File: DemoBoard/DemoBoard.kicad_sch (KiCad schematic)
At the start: 58 parts, among them J1 USB4110GFA, J2 Conn_01x10_Pin, J3 Conn_01x10_Pin, J4 Conn_01x10_Pin, J5 Conn_01x10_Pin, SW1 SW_Push, SW2 SW_Push, U1 RP2040, U2 W25Q128JVSIM, U3 MCP2518FDT-E_QBB, U4 TCAN332DCNR, U5 TLV75533PDBVR, Y1 ABM8-272-T3, Y2 ABM8-20.000MHZ-10-B1U-T

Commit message: Merging v0.1 to main (#1)
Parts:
- removed J2, J3, J4, J5: Conn_01x10_Pin, Connector_PinSocket_2.54mm:PinSocket_1x10_P2.54mm_Vertical, symbol Connector:Conn_01x10_Pin
- removed JP1: 3, Jumper:SolderJumper-2_P1.3mm_Open_RoundedPad1.0x1.5mm, symbol Jumper:SolderJumper_2_Open
- removed JP2: 2, Jumper:SolderJumper-2_P1.3mm_Open_RoundedPad1.0x1.5mm, symbol Jumper:SolderJumper_2_Open
- removed JP3: 1, Jumper:SolderJumper-2_P1.3mm_Open_RoundedPad1.0x1.5mm, symbol Jumper:SolderJumper_2_Open
- removed JP4: 0, Jumper:SolderJumper-2_P1.3mm_Open_RoundedPad1.0x1.5mm, symbol Jumper:SolderJumper_2_Open
- added C24: 100nF, Capacitor_SMD:C_0402_1005Metric_Pad0.74x0.62mm_HandSolder, symbol Device:C
- added C25: 47uF, Capacitor_SMD:C_1206_3216Metric_Pad1.33x1.80mm_HandSolder, symbol Device:C
- added J6: M55-7101242R, inspireFly:HARWIN_M55-7101242R, symbol inspireFly:M55-7101242R
- added J7: MSD-1-A, inspireFly:CUI_MSD-1-A, symbol inspireFly:MSD-1-A
- added J8: Conn_01x17_Pin, Connector_PinSocket_2.54mm:PinSocket_1x17_P2.54mm_Vertical, symbol Connector:Conn_01x17_Pin
- added R11: 10k, Resistor_SMD:R_0402_1005Metric_Pad0.72x0.64mm_HandSolder, symbol Device:R_US
- C22: footprint Capacitor_SMD:C_0402_1005Metric -> Capacitor_SMD:C_0402_1005Metric_Pad0.74x0.62mm_HandSolder
- C23: value 10uF -> 47uF; footprint Capacitor_SMD:C_0402_1005Metric -> Capacitor_SMD:C_1206_3216Metric_Pad1.33x1.80mm_HandSolder
- JP5: value SolderJumper_2_Open -> 3.3V EN; footprint Jumper:SolderJumper-2_P1.3mm_Open_RoundedPad1.0x1.5mm -> inspireFly:SmallJumper
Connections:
- net +3.3V: now also C24.1, J6.B1, J6.B2, J6.B3, J7.4 (VDD), J8.3 (Pin_3), R11.1
- net ADC_0: now also J8.8 (Pin_8)
- net ADC_1: now also J8.9 (Pin_9)
- net ADC_2: now also J8.10 (Pin_10)
- net ADC_3: now also J8.11 (Pin_11)
- net CAN_HIGH: now also J6.A1, J8.2 (Pin_2)
- net CAN_LOW: now also J6.A2, J8.1 (Pin_1)
- net GPIO_14: now also J8.13 (Pin_13)
- net GPIO_15: now also J8.14 (Pin_14)
- net GPIO_16: now also J8.15 (Pin_15)
- net GPIO_17: now also J8.16 (Pin_16)
- net GPIO_6: now also R8.1
- net GPIO_9: now also J8.12 (Pin_12)
- net SPI0_CLK: now also J7.5 (CLK)
- net SPI0_MISO: now also J7.7 (DAT0)
- net SPI0_MOSI: now also J7.3 (CMD)
- net SWCLK: now also J8.4 (Pin_4)
- net SWD: now also J8.6 (Pin_6)
- net VBUS: now also J8.7 (Pin_7)
- net GND renamed COVER_GND
- net COVER_GND: now also C24.2, C25.2, J6.A3, J6.A4, J6.A5, J6.A6, J6.SH1, J6.SH2, J6.SH3, J6.SH4, J7.6 (VSS), J7.G1 (COVER_GND), J7.G2 (COVER_GND), J7.G3 (COVER_GND), J7.G4 (COVER_GND), J8.17 (Pin_17), J8.5 (Pin_5)
- net GPIO_5_DEBUGLED renamed SPI0_CS_SDCARD
- net SPI0_CS_SDCARD: now also J7.2 (CD/DAT3), R11.2; no longer R8.1
- net SPI0_CS renamed SPI0_CS_CAN
- new net BATTERY_VOLTAGE: C25.1, J6.B4, J6.B5, J6.B6
- no-connect marks 5 -> 8
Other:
- note added: "4.2V max voltage"
- note added: "Board Connector"
- note added: "Debug LEDs"
- note added: "Ground unused ADC pins"
- note added: "SD Card"
- note added: "Test Pinout"
- note removed: "Debug + Pinout"
- note removed: "Ground by soldering jumper if not using ADC pin"
- moved on the sheet: C12, C16, C23, CR1, D1, D2, J1, R1, R6, R7, R8, R9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

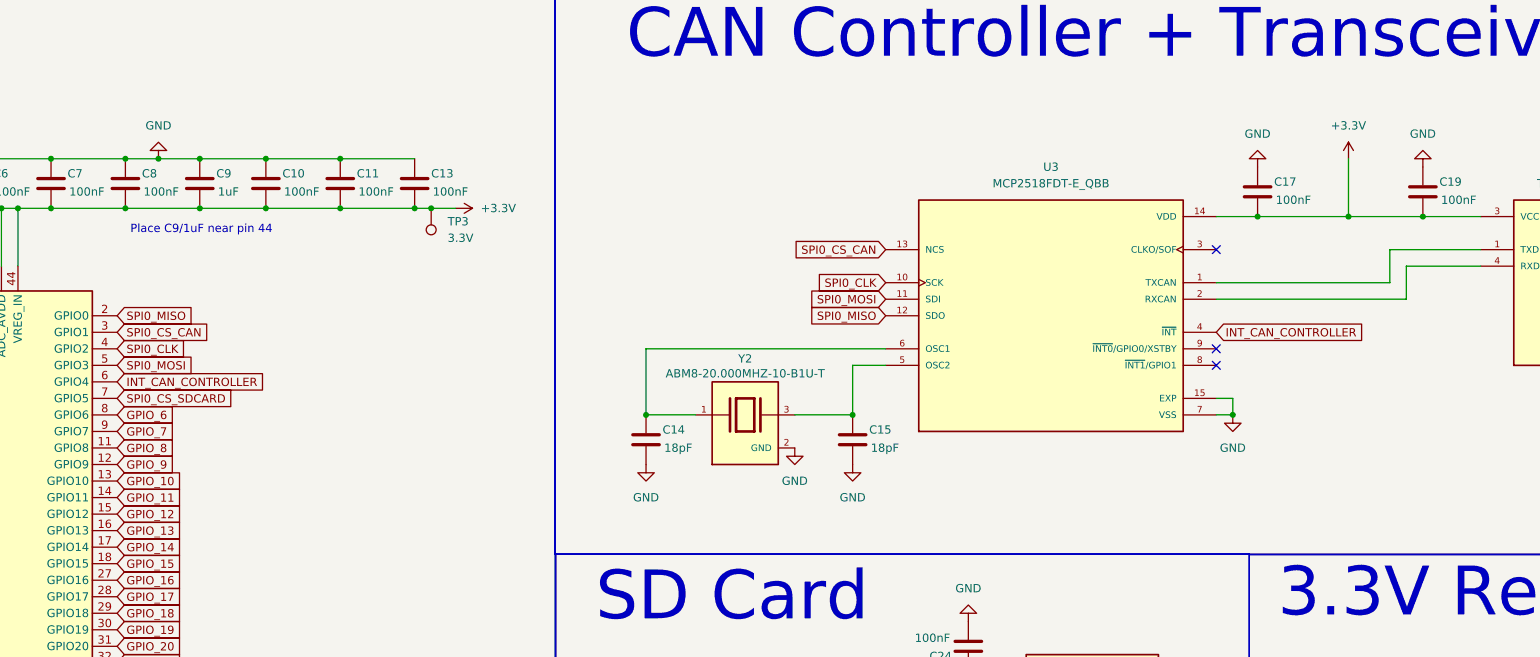
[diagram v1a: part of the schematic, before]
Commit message: Updated DemoBoard to V0.2
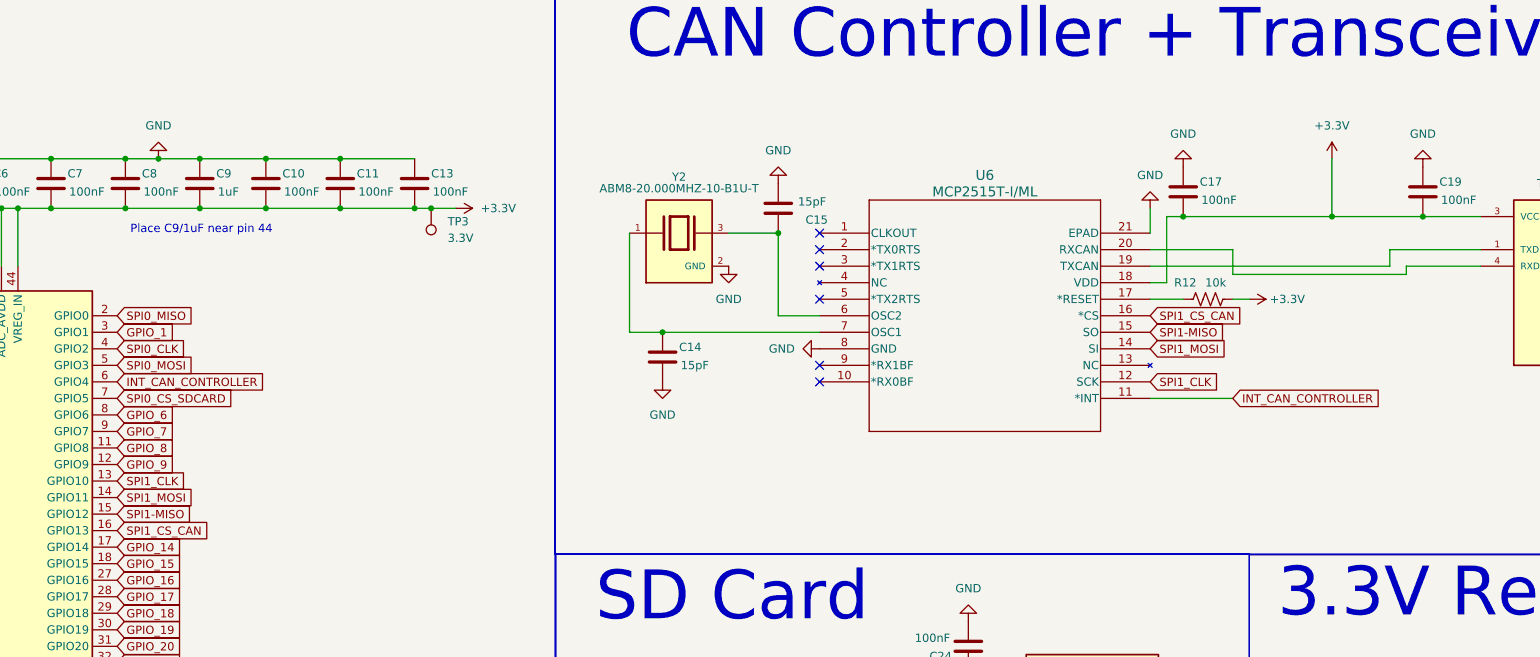
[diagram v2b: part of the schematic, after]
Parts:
- removed U3: MCP2518FDT-E_QBB, inspireFly:SON65P450X300X90-15N, symbol inspireFly:MCP2518FDT-E_QBB
- added R12: 10k, Resistor_SMD:R_0402_1005Metric_Pad0.72x0.64mm_HandSolder, symbol Device:R_US
- added U6: MCP2515T-I/ML, inspireFly:QFN20_4x4MC_MCH, symbol inspireFly:MCP2515T-I_ML
- C14, C15: value 18pF -> 15pF
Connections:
- net +3.3V: now also R12.1, U6.18 (VDD)
- net COVER_GND: now also U6.21 (EPAD), U6.8 (GND)
- net INT_CAN_CONTROLLER: now also U6.11 (*INT)
- net at C14.1, Y2.1: now also U6.7 (OSC1)
- net at C15.1, Y2.3: now also U6.6 (OSC2)
- net at U4.1 (TXD): now also U6.19 (TXCAN)
- net at U4.4 (RXD): now also U6.20 (RXCAN)
- net GPIO_10 renamed SPI1_CLK
- net SPI1_CLK: now also U6.12 (SCK)
- net GPIO_11 renamed SPI1_MOSI
- net SPI1_MOSI: now also U6.14 (SI)
- net GPIO_12 renamed SPI1-MISO
- net SPI1-MISO: now also U6.15 (SO)
- net GPIO_13 renamed SPI1_CS_CAN
- net SPI1_CS_CAN: now also U6.16 (*CS)
- net SPI0_CS_CAN renamed GPIO_1
- new net: R12.2, U6.17 (*RESET)
- no-connect marks 8 -> 11
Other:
- moved on the sheet: C14, C15, C17
